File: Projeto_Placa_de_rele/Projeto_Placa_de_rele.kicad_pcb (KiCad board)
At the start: 2 copper layers, 8 parts, among them J1 Conn_01x03, J2 Screw_Terminal_01x03, K1 SRD-05VDC-SL-C, Q1 BC547

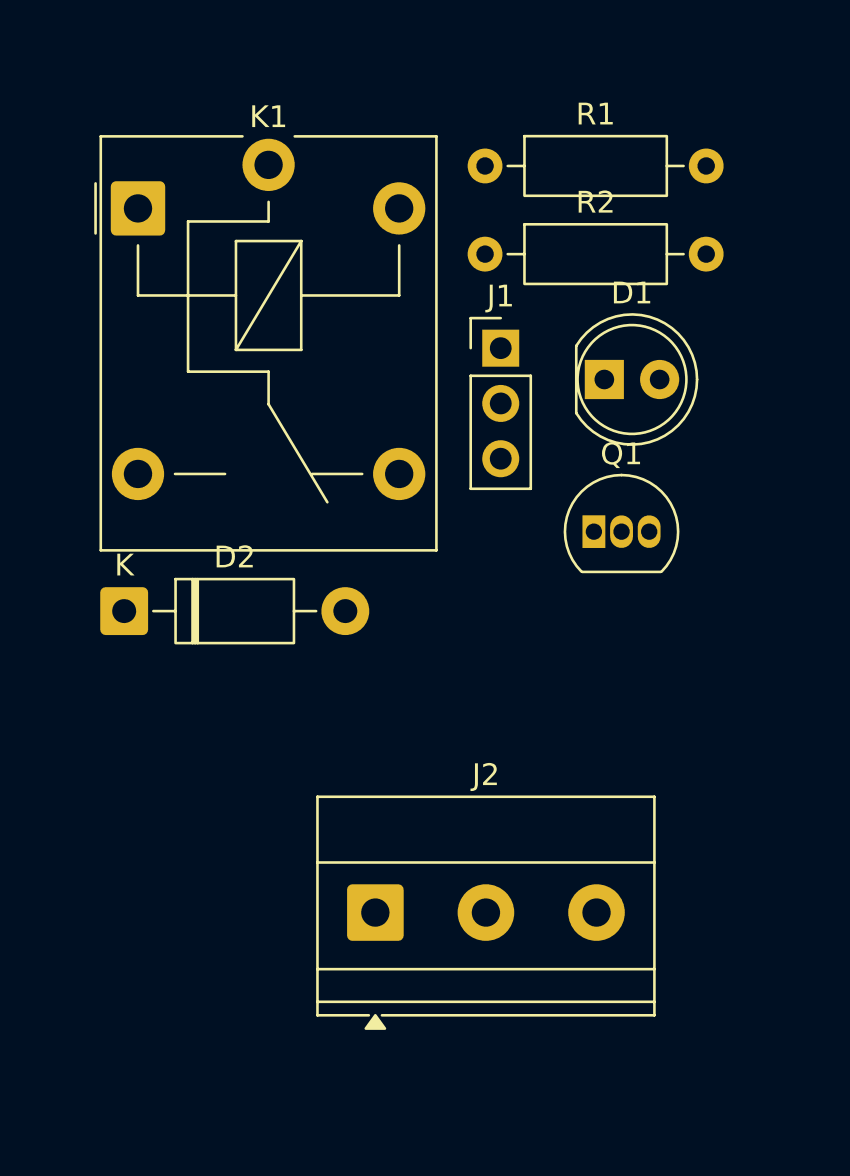
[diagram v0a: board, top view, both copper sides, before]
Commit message: Atualização
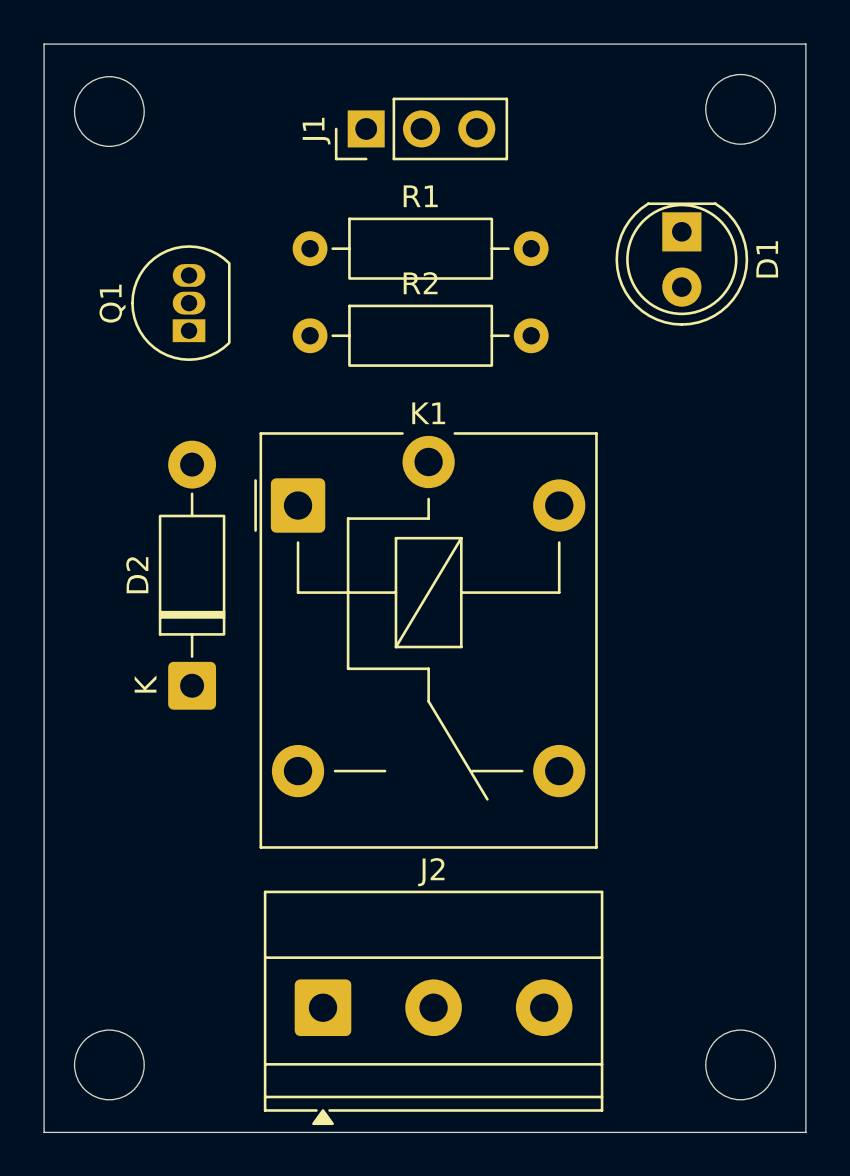
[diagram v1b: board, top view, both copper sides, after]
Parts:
- moved Q1 20.8 mm to (133.9, 93.3), turned to 90 degrees
- moved K1 15.5 mm to (138.9, 101.3)
- moved J1 11.8 mm to (142.0, 84.0), turned to 90 degrees
- moved R1 8.89 mm to (139.4, 89.5)
- moved R2 8.87 mm to (139.4, 93.5)
- moved D1 7.66 mm to (156.5, 88.7), turned to -90 degrees
- moved J2 4.99 mm to (140.0, 124.4)
- moved D2 4.64 mm to (134.0, 109.6), turned to 90 degrees
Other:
- board outline added: 35 x 50 mm
